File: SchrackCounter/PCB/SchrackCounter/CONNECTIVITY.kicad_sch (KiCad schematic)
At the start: 23 parts, among them J1 TYPE-C-31-M-12, U8 USBLC6-2SC6

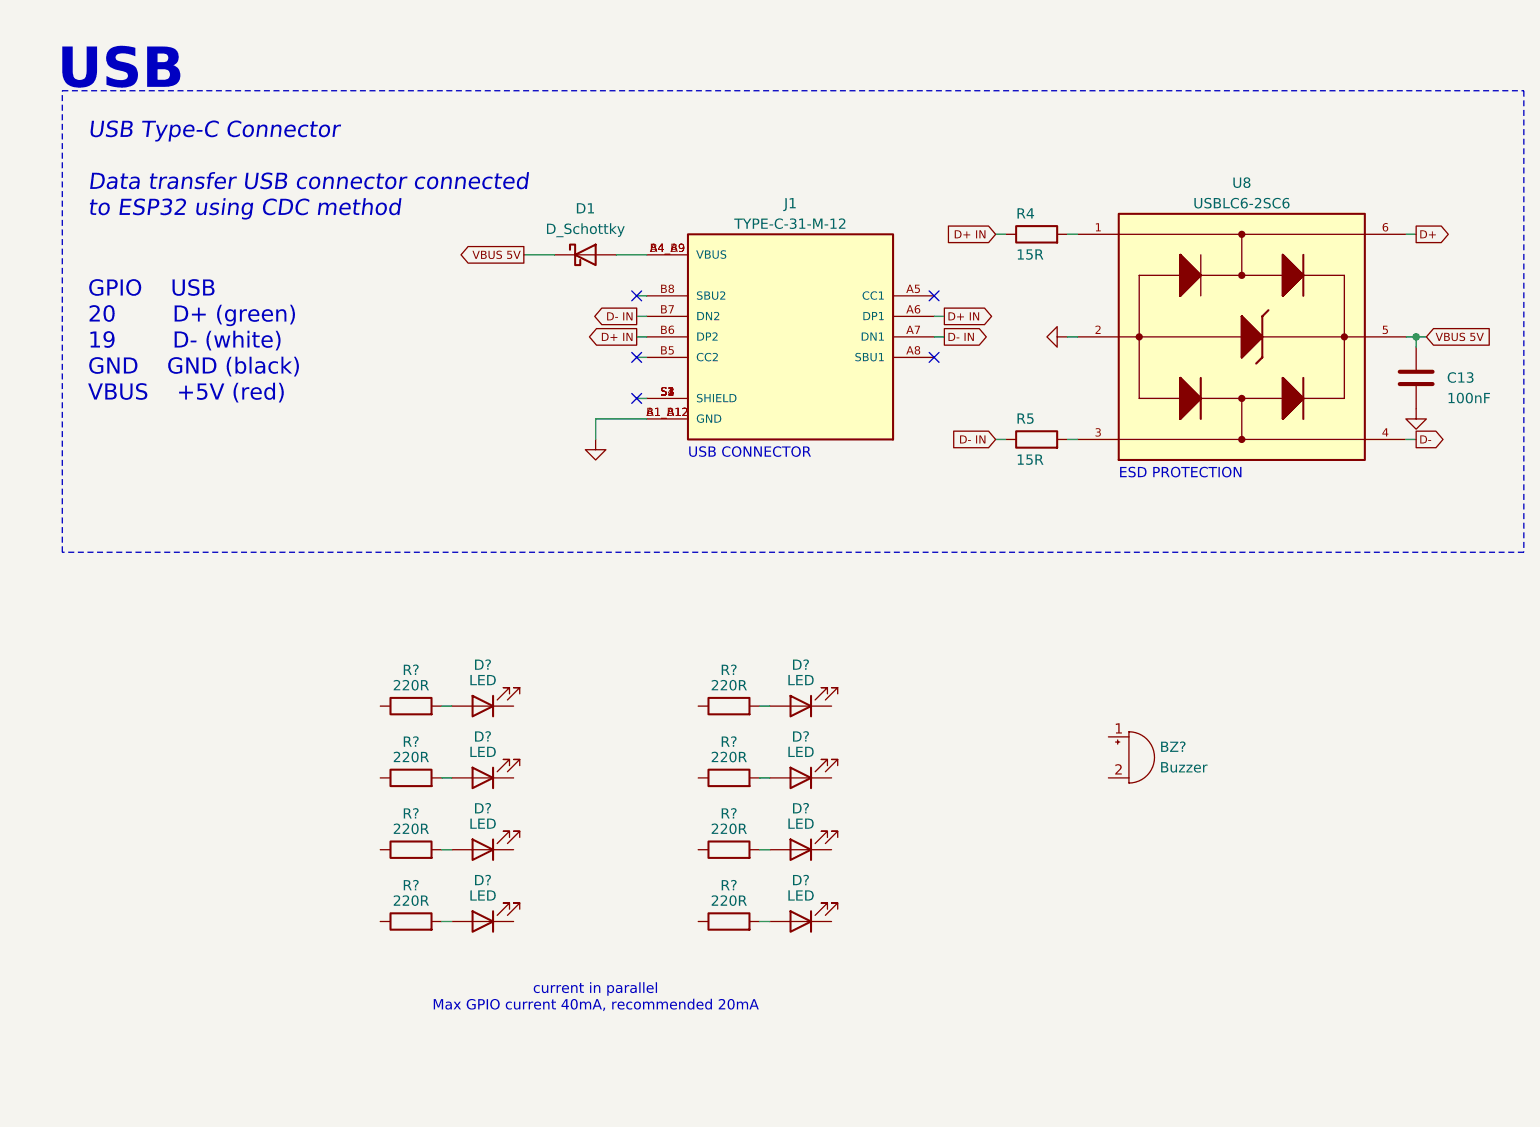
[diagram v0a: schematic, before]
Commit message: sleep, overated imo
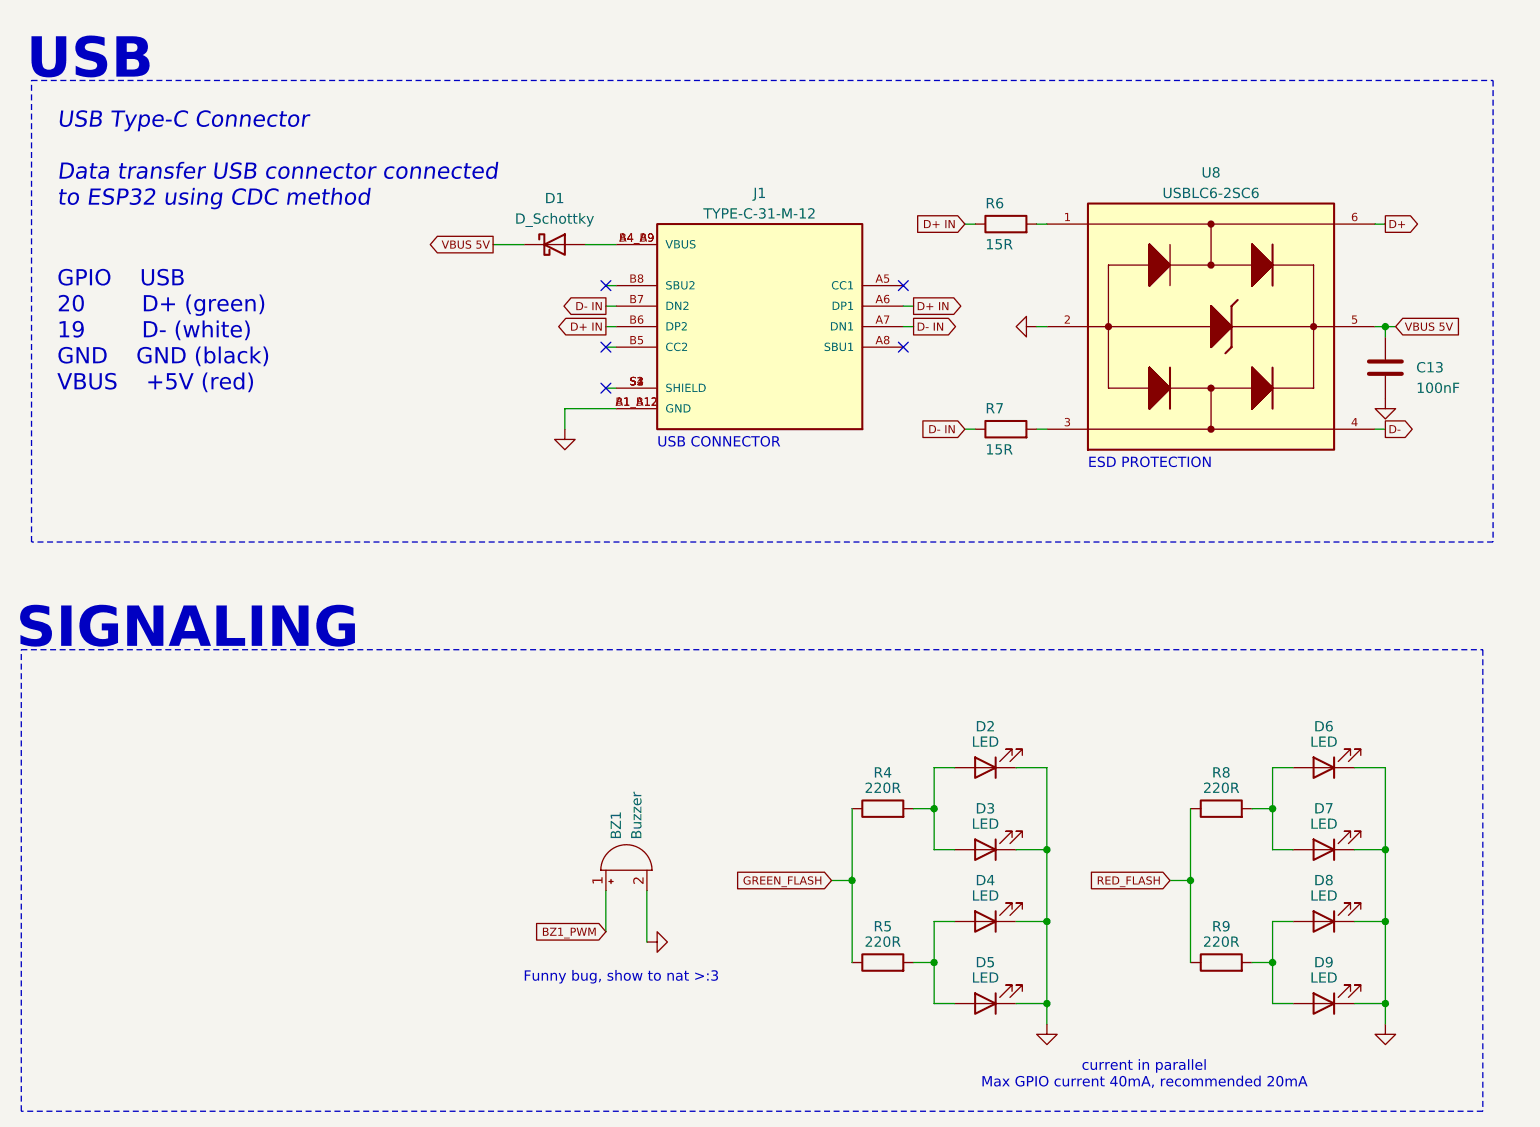
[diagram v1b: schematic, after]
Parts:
- removed D? (x4): LED, symbol Device:LED
- removed R? (x8): 220R, symbol Device:R
- added D6, D7, D8, D9: LED, LED_SMD:LED_0805_2012Metric_Pad1.15x1.40mm_HandSolder, symbol Device:LED
- added R4, R5, R8, R9: 220R, Resistor_SMD:R_0805_2012Metric_Pad1.20x1.40mm_HandSolder, symbol Device:R
- BZ1: renamed from BZ?; footprint (none) -> Schrack_brd:CUI_CPT-1625-80
- D2, D3, D4, D5: renamed from D?; footprint (none) -> LED_SMD:LED_0805_2012Metric_Pad1.15x1.40mm_HandSolder
- renumbered R4 to R6, R5 to R7
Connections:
- net GND: now also BZ1.2 (-), D2.1 (K), D3.1 (K), D4.1 (K), D5.1 (K), D6.1 (K), D7.1 (K), D8.1 (K), D9.1 (K)
- net at D4.2 (A): now also D5.2 (A), R5.2
- net BZ1_PWM: now reaches BZ1.1 (+)
- net at D2.2 (A): now also D3.2 (A), R4.2
- new net: D6.2 (A), D7.2 (A), R8.2
- new net: D8.2 (A), D9.2 (A), R9.2
- new net GREEN_FLASH: R4.1, R5.1
- new net RED_FLASH: R8.1, R9.1
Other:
- note added: "Funny bug, show to nat >:3"
- note added: "SIGNALING"
- moved on the sheet: BZ1, C13, D1, D2, D3, D4, D5, J1, R6, R7, U8
